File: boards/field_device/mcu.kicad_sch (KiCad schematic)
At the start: 19 parts, among them J1 Conn_01x05_Pin, J2 Conn_01x02_Pin, SW1 SW_SPST, U2 STM32C011F6Px

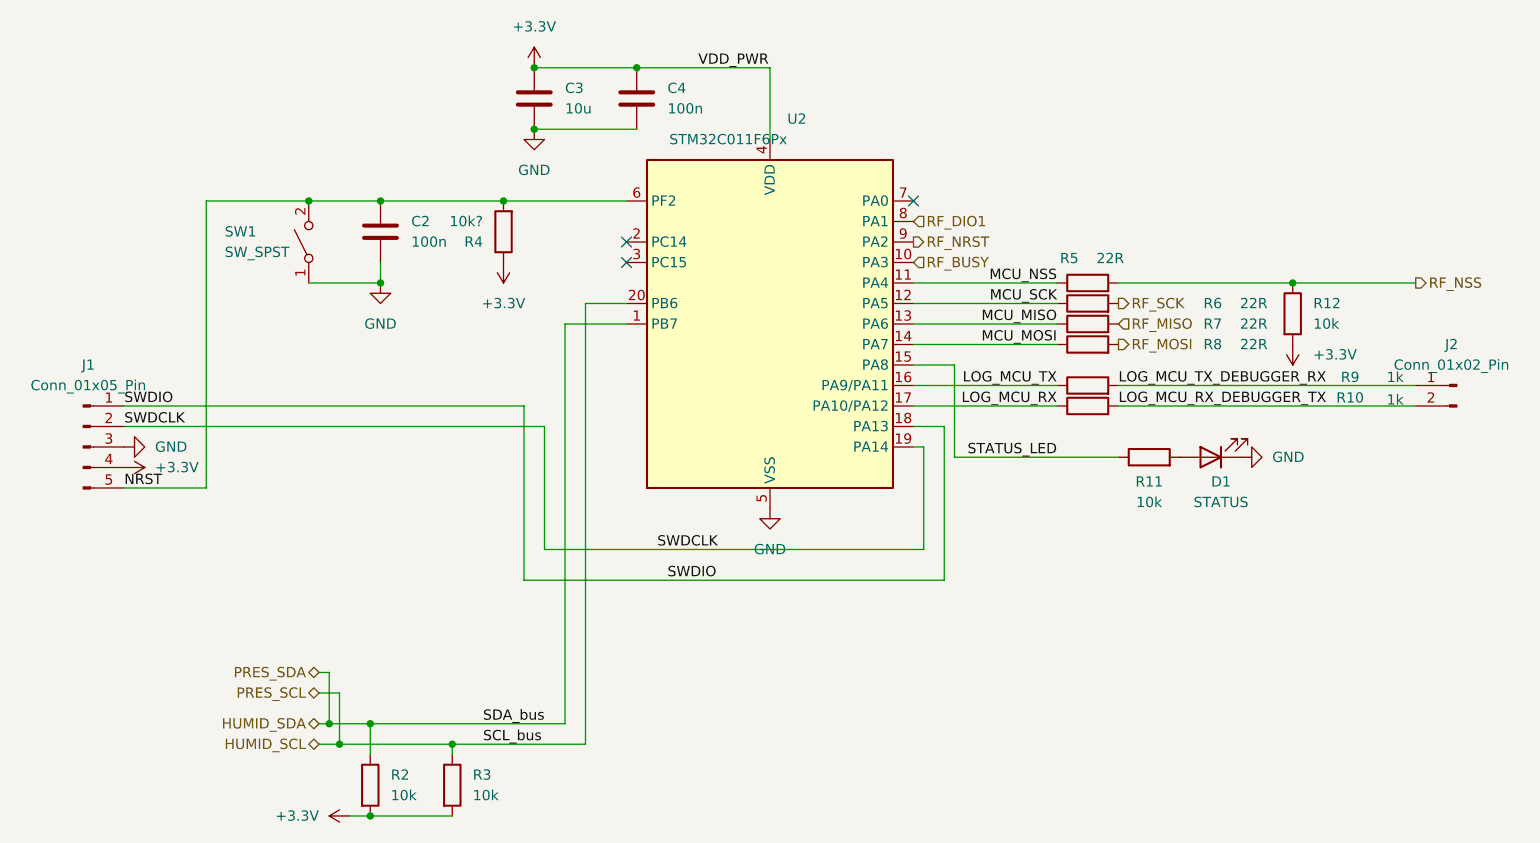
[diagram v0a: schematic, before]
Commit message: rrev 4
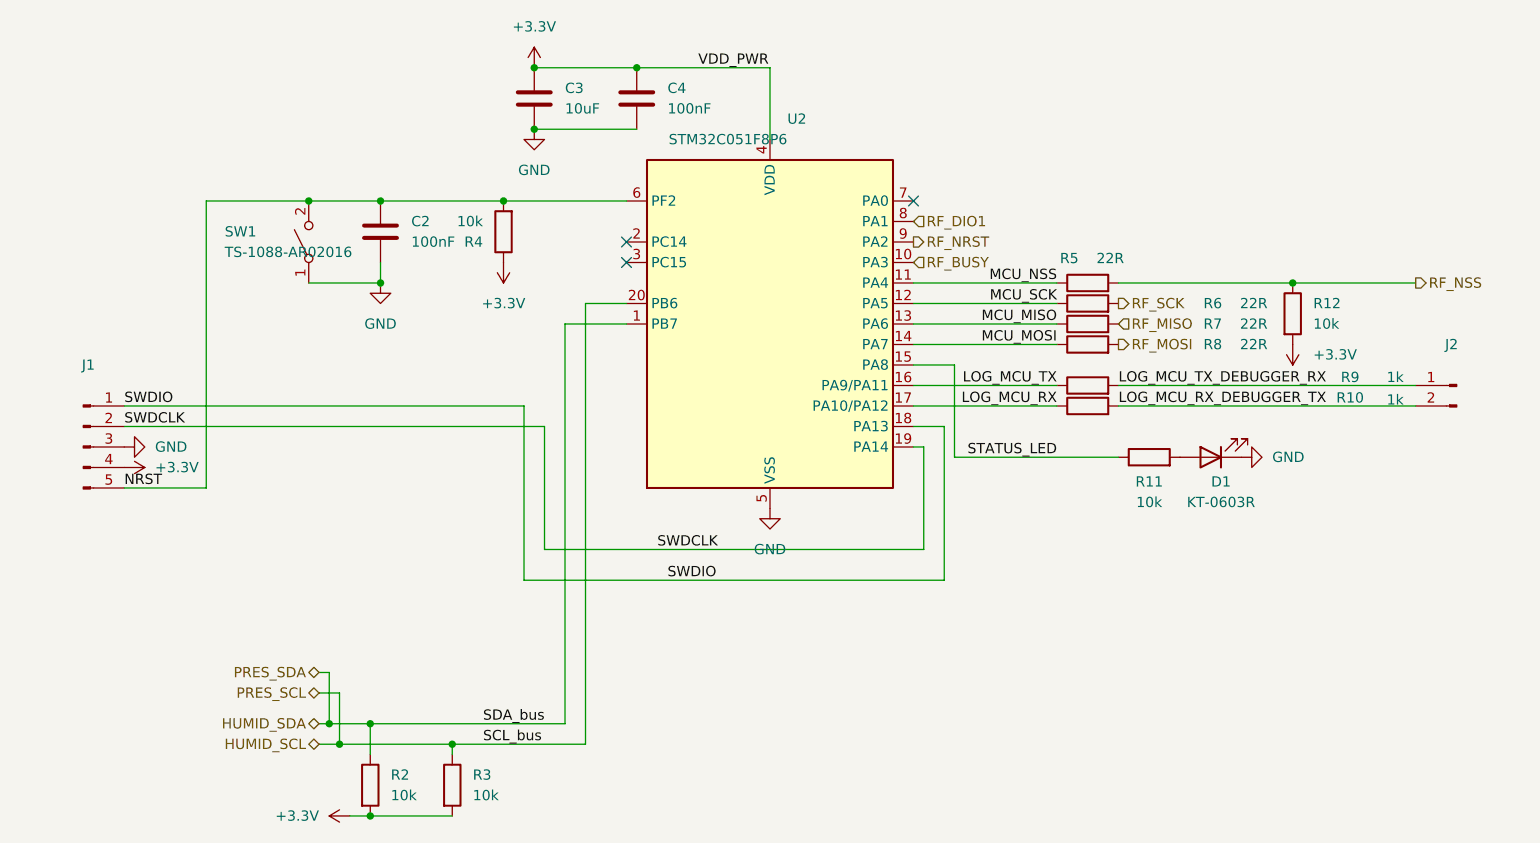
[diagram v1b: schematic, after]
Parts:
- C2, C4: value 100n -> 100nF
- C3: value 10u -> 10uF
- D1: value STATUS -> KT-0603R
- J1: value Conn_01x05_Pin -> (none); footprint Connector_PinHeader_1.00mm:PinHeader_1x05_P1.00mm_Vertical -> Connector_PinHeader_2.54mm:PinHeader_1x05_P2.54mm_Vertical
- J2: value Conn_01x02_Pin -> (none); footprint Connector_PinHeader_1.00mm:PinHeader_1x02_P1.00mm_Vertical -> Connector_PinHeader_2.54mm:PinHeader_1x02_P2.54mm_Vertical
- R3: footprint Resistor_SMD:R_0603_1608Metric_Pad0.98x0.95mm_HandSolder -> Resistor_SMD:R_0402_1005Metric_Pad0.72x0.64mm_HandSolder
- R4: value 10k? -> 10k
- SW1: value SW_SPST -> TS-1088-AR02016; footprint UnEasy-LCSC:KEY-SMD_L3.9-W3.0-LS5.0-EH -> UnEasy-LCSC:SW-SMD_L3.9-W3.0-P4.45
- U2: value STM32C011F6Px -> STM32C051F8P6
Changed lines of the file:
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@@
 			)
 		)
-		(property "Value" "Conn_01x05_Pin"
+		(property "Value" ""
 			(at 42.545 67.31 0)
 			(show_name no)
@@
 			)
 		)
-		(property "Footprint" "Connector_PinHeader_1.00mm:PinHeader_1x05_P1.00mm_Vertical"
+		(property "Footprint" "Connector_PinHeader_2.54mm:PinHeader_1x05_P2.54mm_Vertical"
 			(at 41.91 74.93 0)
 			(hide yes)
@@
 			)
 		)
-		(property "Value" "STM32C011F6Px"
+		(property "Value" "STM32C051F8P6"
 			(at 129.1433 36.83 0)
 			(show_name no)
@@
 			)
 		)
-		(property "Value" "100n"
+		(property "Value" "100nF"
 			(at 114.3 33.0199 0)
 			(show_name no)
@@
 			)
 		)
-		(property "Value" "10k?"
+		(property "Value" "10k"
 			(at 91.44 46.9901 0)
 			(show_name no)
@@
 			)
 		)
-		(property "Value" "100n"
+		(property "Value" "100nF"
 			(at 82.55 49.5299 0)
 			(show_name no)
@@
 			)
 		)
-		(property "Value" "SW_SPST"
+		(property "Value" "TS-1088-AR02016"
 			(at 59.436 50.8 90)
 			(show_name no)
@@
 			)
 		)
-		(property "Footprint" "UnEasy-LCSC:KEY-SMD_L3.9-W3.0-LS5.0-EH"
+		(property "Footprint" "UnEasy-LCSC:SW-SMD_L3.9-W3.0-P4.45"
 			(at 69.85 49.53 0)
 			(hide yes)
@@
 			)
 		)
-		(property "Value" "Conn_01x02_Pin"
+		(property "Value" ""
 			(at 211.455 64.77 0)
 			(show_name no)
@@
 			)
 		)
-		(property "Footprint" "Connector_PinHeader_1.00mm:PinHeader_1x02_P1.00mm_Vertical"
+		(property "Footprint" "Connector_PinHeader_2.54mm:PinHeader_1x02_P2.54mm_Vertical"
 			(at 212.09 67.31 0)
 			(hide yes)
@@
 			)
 		)
-		(property "Value" "10u"
+		(property "Value" "10uF"
 			(at 101.6 33.0199 0)
 			(show_name no)
@@
 			)
 		)
-		(property "Value" "STATUS"
+		(property "Value" "KT-0603R"
 			(at 182.88 81.788 0)
 			(show_name no)
@@
 			)
 		)
-		(property "Footprint" "Resistor_SMD:R_0603_1608Metric_Pad0.98x0.95mm_HandSolder"
+		(property "Footprint" "Resistor_SMD:R_0402_1005Metric_Pad0.72x0.64mm_HandSolder"
 			(at 85.852 116.84 90)
 			(hide yes)

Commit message: Revert "rrev 4"
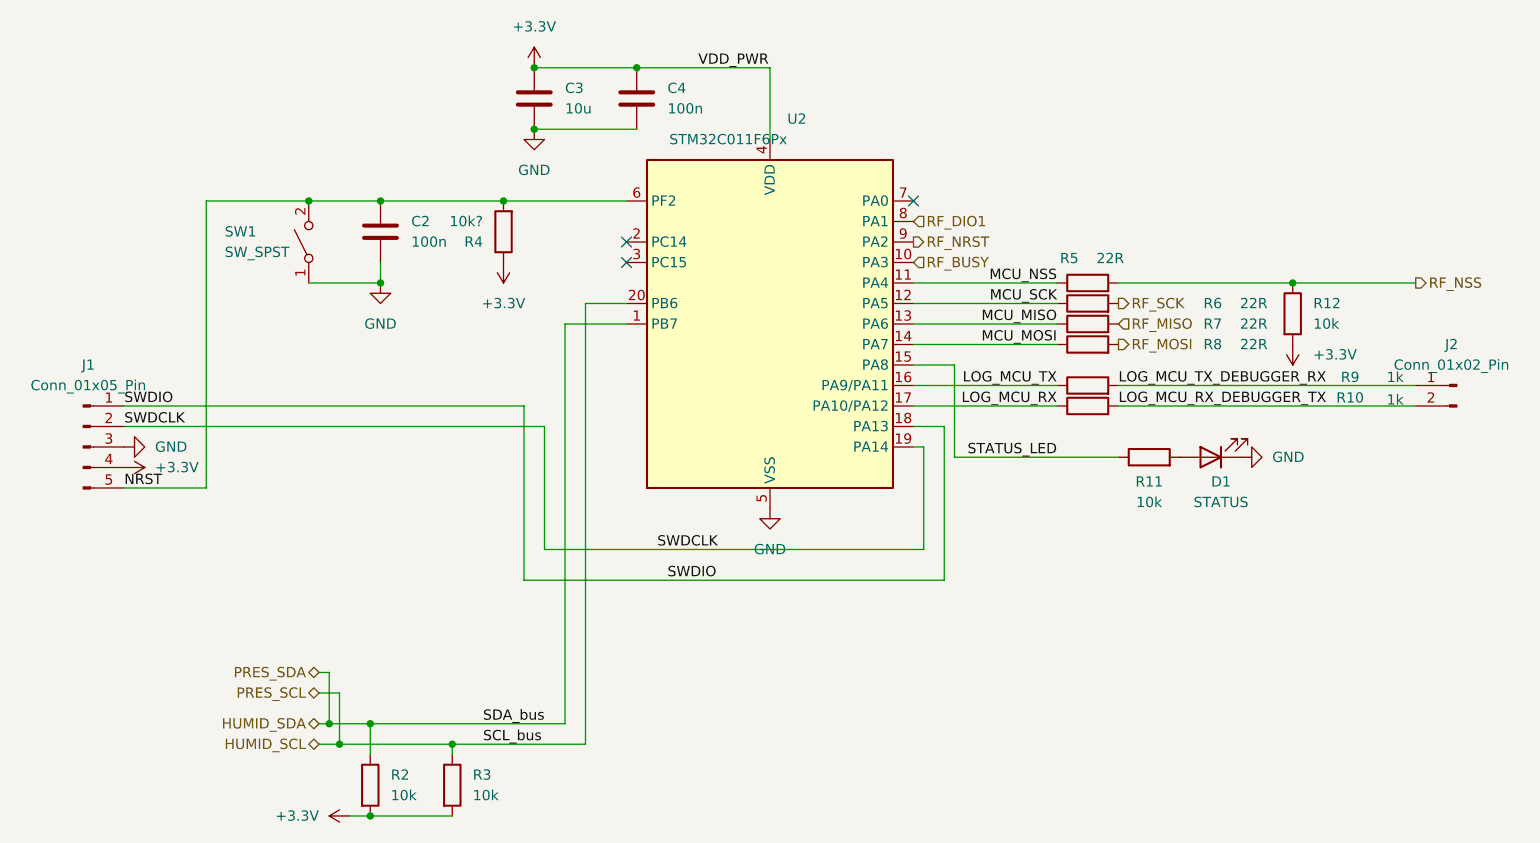
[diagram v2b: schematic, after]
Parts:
- C2, C4: value 100nF -> 100n
- C3: value 10uF -> 10u
- D1: value KT-0603R -> STATUS
- J1: value (none) -> Conn_01x05_Pin; footprint Connector_PinHeader_2.54mm:PinHeader_1x05_P2.54mm_Vertical -> Connector_PinHeader_1.00mm:PinHeader_1x05_P1.00mm_Vertical
- J2: value (none) -> Conn_01x02_Pin; footprint Connector_PinHeader_2.54mm:PinHeader_1x02_P2.54mm_Vertical -> Connector_PinHeader_1.00mm:PinHeader_1x02_P1.00mm_Vertical
- R3: footprint Resistor_SMD:R_0402_1005Metric_Pad0.72x0.64mm_HandSolder -> Resistor_SMD:R_0603_1608Metric_Pad0.98x0.95mm_HandSolder
- R4: value 10k -> 10k?
- SW1: value TS-1088-AR02016 -> SW_SPST; footprint UnEasy-LCSC:SW-SMD_L3.9-W3.0-P4.45 -> UnEasy-LCSC:KEY-SMD_L3.9-W3.0-LS5.0-EH
- U2: value STM32C051F8P6 -> STM32C011F6Px
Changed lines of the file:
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@@
 			)
 		)
-		(property "Value" ""
+		(property "Value" "Conn_01x05_Pin"
 			(at 42.545 67.31 0)
 			(show_name no)
@@
 			)
 		)
-		(property "Footprint" "Connector_PinHeader_2.54mm:PinHeader_1x05_P2.54mm_Vertical"
+		(property "Footprint" "Connector_PinHeader_1.00mm:PinHeader_1x05_P1.00mm_Vertical"
 			(at 41.91 74.93 0)
 			(hide yes)
@@
 			)
 		)
-		(property "Value" "STM32C051F8P6"
+		(property "Value" "STM32C011F6Px"
 			(at 129.1433 36.83 0)
 			(show_name no)
@@
 			)
 		)
-		(property "Value" "100nF"
+		(property "Value" "100n"
 			(at 114.3 33.0199 0)
 			(show_name no)
@@
 			)
 		)
-		(property "Value" "10k"
+		(property "Value" "10k?"
 			(at 91.44 46.9901 0)
 			(show_name no)
@@
 			)
 		)
-		(property "Value" "100nF"
+		(property "Value" "100n"
 			(at 82.55 49.5299 0)
 			(show_name no)
@@
 			)
 		)
-		(property "Value" "TS-1088-AR02016"
+		(property "Value" "SW_SPST"
 			(at 59.436 50.8 90)
 			(show_name no)
@@
 			)
 		)
-		(property "Footprint" "UnEasy-LCSC:SW-SMD_L3.9-W3.0-P4.45"
+		(property "Footprint" "UnEasy-LCSC:KEY-SMD_L3.9-W3.0-LS5.0-EH"
 			(at 69.85 49.53 0)
 			(hide yes)
@@
 			)
 		)
-		(property "Value" ""
+		(property "Value" "Conn_01x02_Pin"
 			(at 211.455 64.77 0)
 			(show_name no)
@@
 			)
 		)
-		(property "Footprint" "Connector_PinHeader_2.54mm:PinHeader_1x02_P2.54mm_Vertical"
+		(property "Footprint" "Connector_PinHeader_1.00mm:PinHeader_1x02_P1.00mm_Vertical"
 			(at 212.09 67.31 0)
 			(hide yes)
@@
 			)
 		)
-		(property "Value" "10uF"
+		(property "Value" "10u"
 			(at 101.6 33.0199 0)
 			(show_name no)
@@
 			)
 		)
-		(property "Value" "KT-0603R"
+		(property "Value" "STATUS"
 			(at 182.88 81.788 0)
 			(show_name no)
@@
 			)
 		)
-		(property "Footprint" "Resistor_SMD:R_0402_1005Metric_Pad0.72x0.64mm_HandSolder"
+		(property "Footprint" "Resistor_SMD:R_0603_1608Metric_Pad0.98x0.95mm_HandSolder"
 			(at 85.852 116.84 90)
 			(hide yes)
